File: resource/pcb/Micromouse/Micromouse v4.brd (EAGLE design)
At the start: 63.8 x 75.3 mm, 8 parts

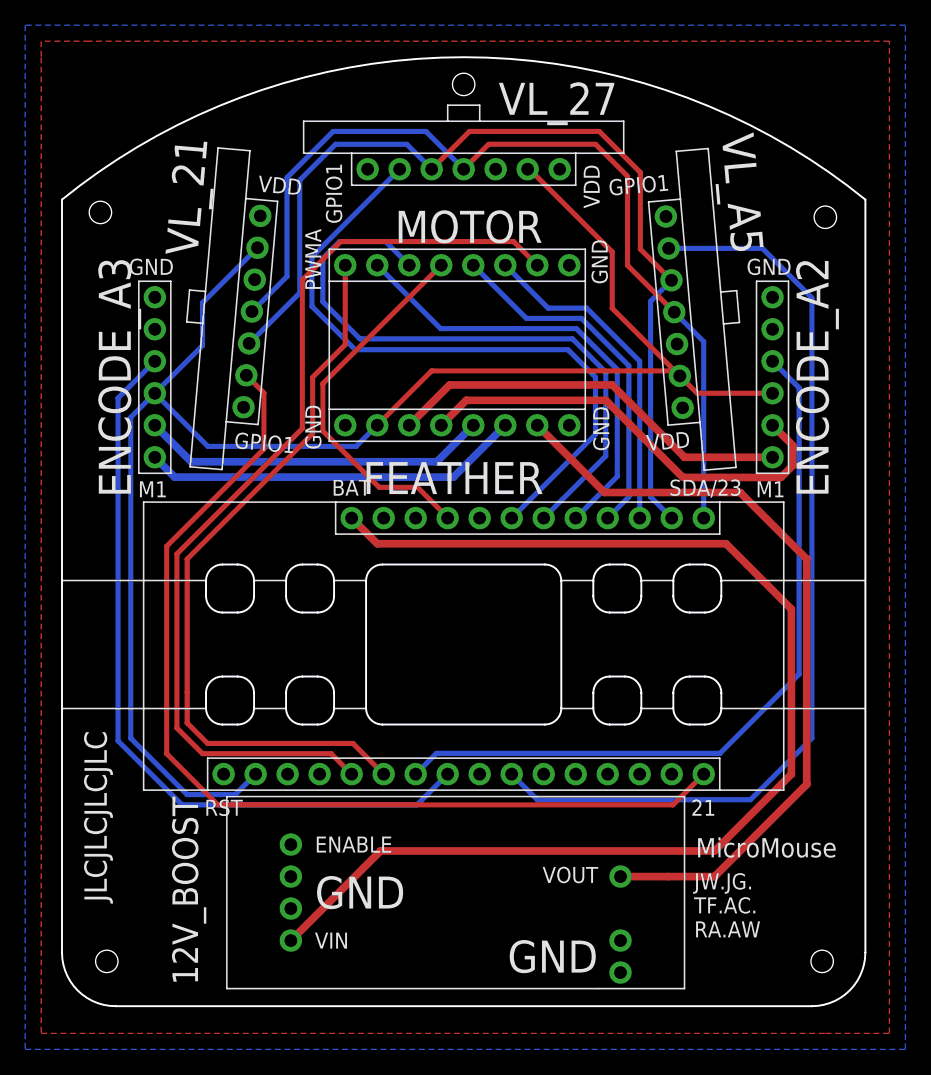
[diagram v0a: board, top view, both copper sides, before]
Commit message: Updated PCB
Signed-off-by: AJ Walter <git@awalter.net>
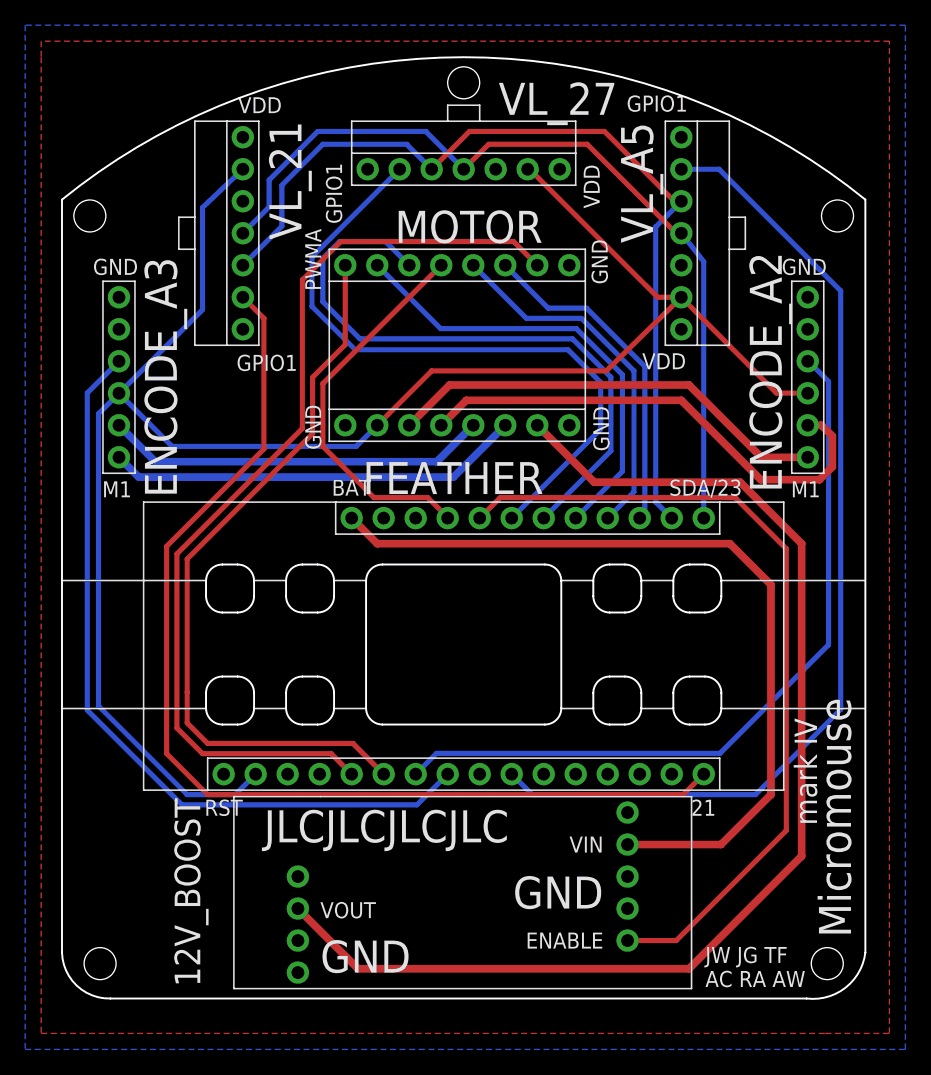
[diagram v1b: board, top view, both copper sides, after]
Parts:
- moved VL_21 6.48 mm to (22.4, 73.7), turned to 180 degrees
- moved VL_A5 6.35 mm to (54.6, 61.0), turned to 0 degrees
- moved 12V_BOOST 3.86 mm to (40.2, 15.0), turned to 180 degrees
- moved ENCODE_A3 2.84 mm to (12.5, 63.5)
- moved ENCODE_A2 2.79 mm to (67.2, 63.5)
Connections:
- new net N$1: 12V_BOOST.EN, ESP1.12/A11
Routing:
- net N$1: track 0.00 -> 65.3 mm
- net BOOST_OUT: track 61.5 -> 95.3 mm
- net BOOST_IN: track 96.2 -> 65.1 mm
- net VCC: track 131.0 -> 144.3 mm
- net N$19: track 79.1 -> 84.8 mm
- net SDA: track 73.1 -> 67.6 mm
- net N$20: track 74.6 -> 79.5 mm
- net SCL: track 76.1 -> 71.5 mm
- net MA2: track 35.5 -> 39.6 mm
- net MB1: track 30.2 -> 33.0 mm
- net MB2: track 27.7 -> 30.5 mm
- net MA1: track 32.5 -> 35.3 mm
- net N$16: track 60.6 -> 61.5 mm
- net N$15: track 59.4 -> 60.2 mm
- net N$11: track 29.8 -> 30.6 mm
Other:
- board size 63.8 x 75.3 mm -> 63.8 x 74.7 mm
- board text added: "JW JG TF AC RA AW"
- board text added: "Micromouse"
- board text added: "mark IV"
- board text removed: "JW.JG. TF.AC. RA.AW"
- board text removed: "MicroMouse"
